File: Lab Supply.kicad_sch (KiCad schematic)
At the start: 56 parts, among them J1 V+, J2 V-, Q1 TIP121, Q2 2N3904, Q3 TIP121, Q5 2N3904, T1 115V to 24V, U1 LM324, U2 MCP4922, U3 LM7805, U4 LM4040DBZ-2.0, U6 MCP3202

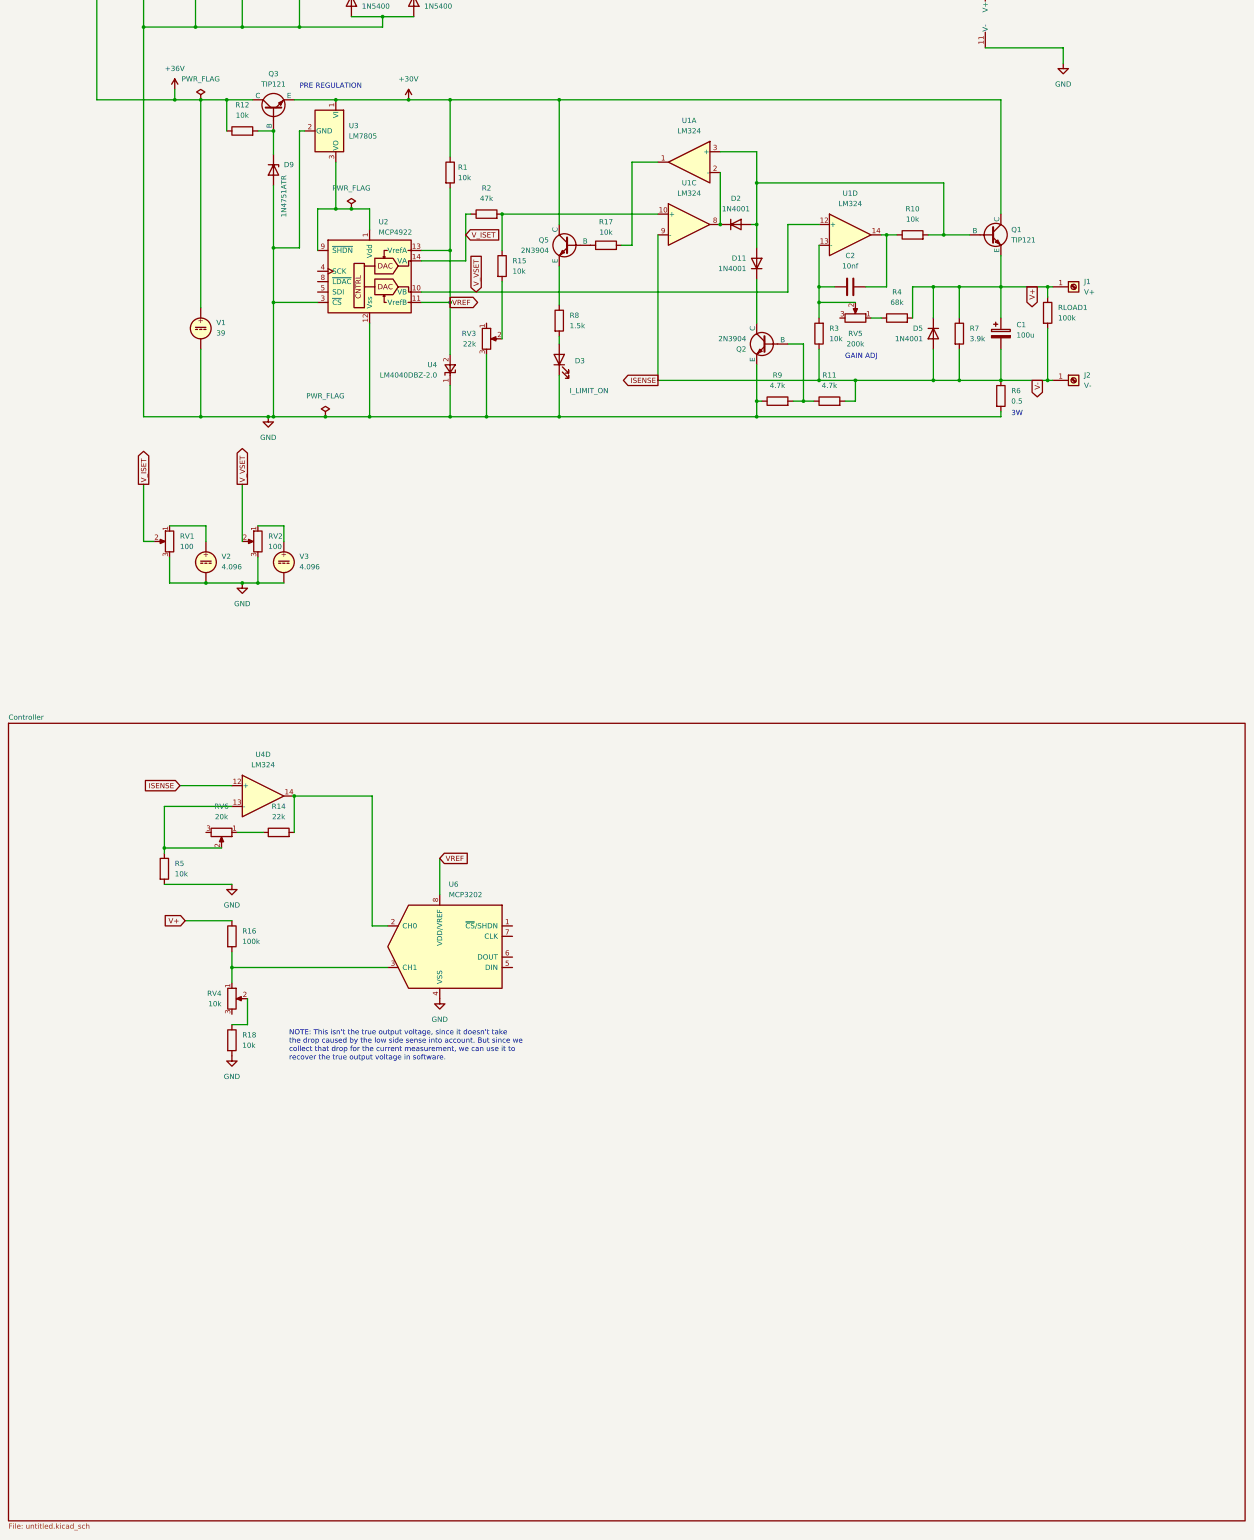
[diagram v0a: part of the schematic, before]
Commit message: Started working on firmware
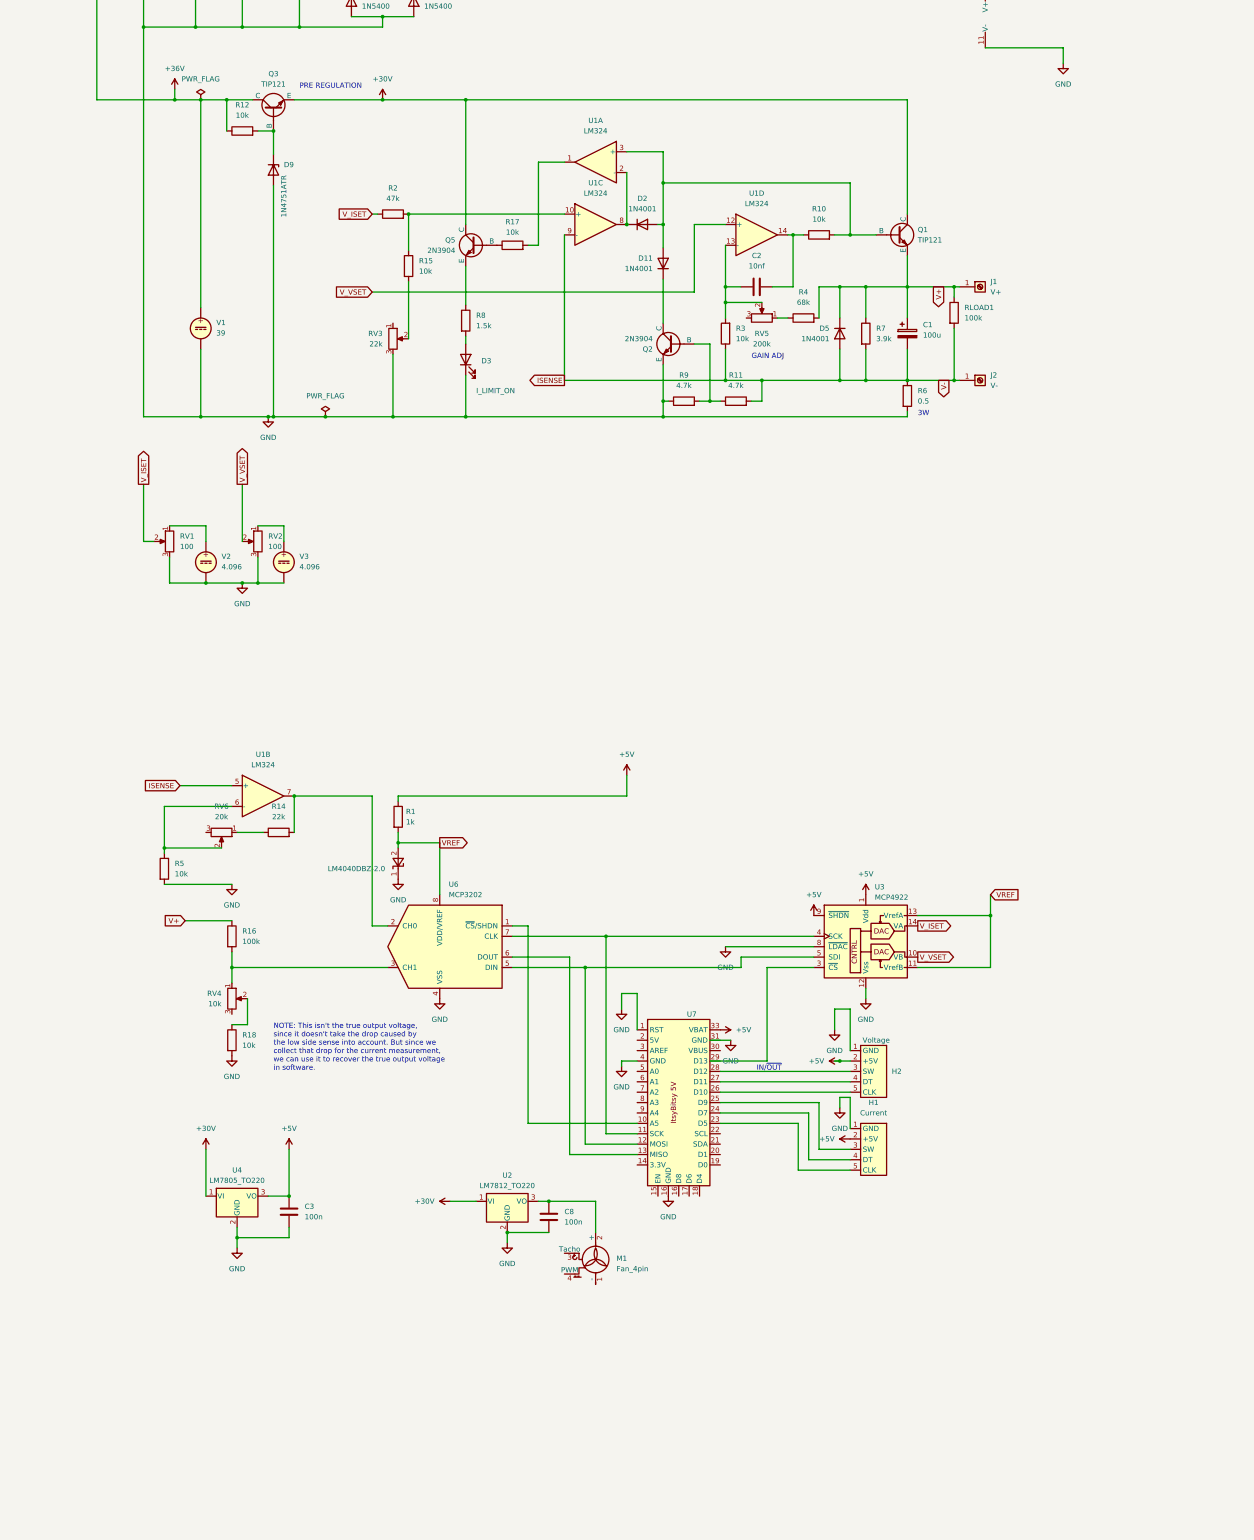
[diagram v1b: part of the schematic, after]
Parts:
- removed U2: MCP4922, Package_DIP:DIP-14_W7.62mm, symbol Analog_DAC:MCP4922
- removed U3: LM7805, Package_TO_SOT_THT:TO-220-3_Vertical, symbol Regulator_Linear:LM7805_TO220
- removed unit 1 of U4
- added C3: 100n, Capacitor_THT:C_Rect_L10.0mm_W2.5mm_P7.50mm_MKS4, symbol Device:C
- added C8: 100n, symbol Device:C
- added H1: Current, symbol Headers:Rotary_Header
- added H2: Voltage, symbol Headers:Rotary_Header
- added M1: Fan_4pin, symbol Motor:Fan_4pin
- added U2: LM7812_TO220, Package_TO_SOT_THT:TO-220-3_Vertical, symbol Regulator_Linear:LM7812_TO220
- added U3: MCP4922, Package_DIP:DIP-14_W7.62mm, symbol Analog_DAC:MCP4922
- added U4: LM7805_TO220, Package_TO_SOT_THT:TO-220-3_Vertical, symbol Regulator_Linear:LM7805_TO220
- added U5: LM4040DBZ-2.0, Package_TO_SOT_SMD:SOT-23, symbol Reference_Voltage:LM4040DBZ-2.0
- added U7: ~, Arduino:Itsy Bitsy 5V, symbol Arduino:ItsyBitsy_32u4-5V
- R1: value 10k -> 1k
- R14, R16, R18, R5: footprint (none) -> Resistor_THT:R_Axial_DIN0207_L6.3mm_D2.5mm_P2.54mm_Vertical
- RV3, RV4, RV6: footprint (none) -> Potentiometer_THT:Potentiometer_Bourns_3339H_Vertical
- RV5: footprint Resistor_THT:R_Axial_DIN0207_L6.3mm_D2.5mm_P2.54mm_Vertical -> Potentiometer_THT:Potentiometer_Bourns_3339H_Vertical
- U1: renamed from U4; footprint (none) -> Package_DIP:DIP-16_W7.62mm
- U6: footprint (none) -> Package_DIP:DIP-8_W7.62mm
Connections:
- net +28V: now also U2.1 (VI), U4.1 (VI); no longer R1.1
- net GND: now also C3.2, C8.2, H1.1 (GND), H2.1 (GND), U2.2 (GND), U3.12 (Vss), U3.8 (~{LDAC}), U4.2 (GND), U5.1 (K), U7.1 (RST), U7.16 (GND), U7.4 (GND)
- net ISENSE: now also U1.5 (+); no longer U1.12 (+)
- net VREF: now also U3.11 (VrefB), U3.13 (VrefA), U5.2 (A)
- net V_ISET: now also U3.14 (VA)
- net V_VSET: now also U3.10 (VB)
- net at R5.1, RV6.2: now also U1.6 (-); no longer U1.13 (-)
- net at R14.2, U6.2 (CH0): now also U1.7; no longer U1.14
- net at U6.1 (~{CS}/SHDN): now also U7.10 (A5)
- net at U6.5 (DIN): now also U3.5 (SDI), U7.12 (MOSI)
- net at U6.6 (DOUT): now also U7.13 (MISO)
- net at U6.7 (CLK): now also U3.4 (SCK), U7.11 (SCK)
- new net: C8.1, M1.2 (+), U2.3 (VO)
- new net: H1.3 (SW), U7.25 (D9)
- new net: H1.4 (DT), U7.24 (D7)
- new net: H1.5 (CLK), U7.23 (D5)
- new net: H2.5 (CLK), U7.26 (D10)
- new net: H2.4 (DT), U7.27 (D11)
- new net: H2.3 (SW), U7.28 (D12)
- new net +5V: C3.1, H1.2 (+5V), H2.2 (+5V), R1.1, U3.1 (Vdd), U3.9 (~{SHDN}), U4.3 (VO), U7.33 (VBAT)
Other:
- removed sheet Controller
- note added: "IN/~{OUT}"
- moved on the sheet: C1, C2, D11, D2, D3, D5, J1, J2, Q1, Q2, Q5, R10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

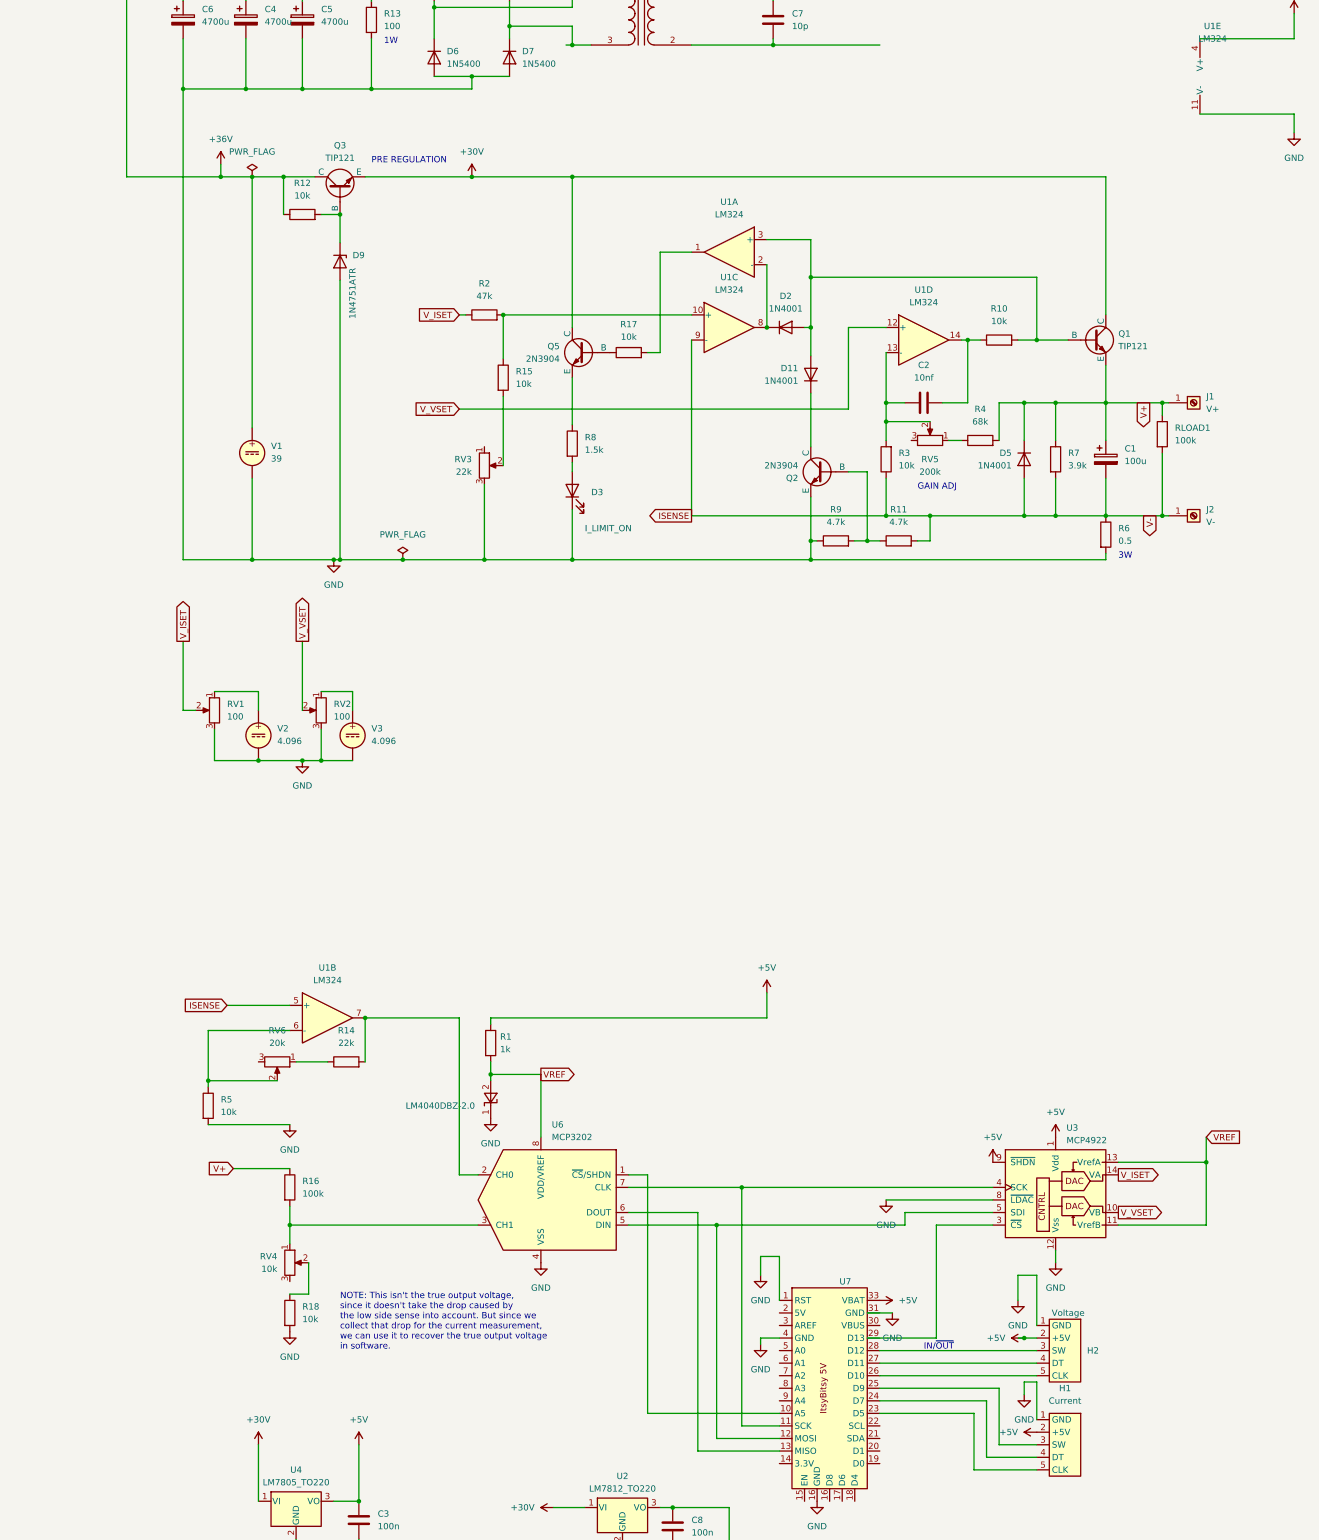
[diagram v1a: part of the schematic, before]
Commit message: WIP
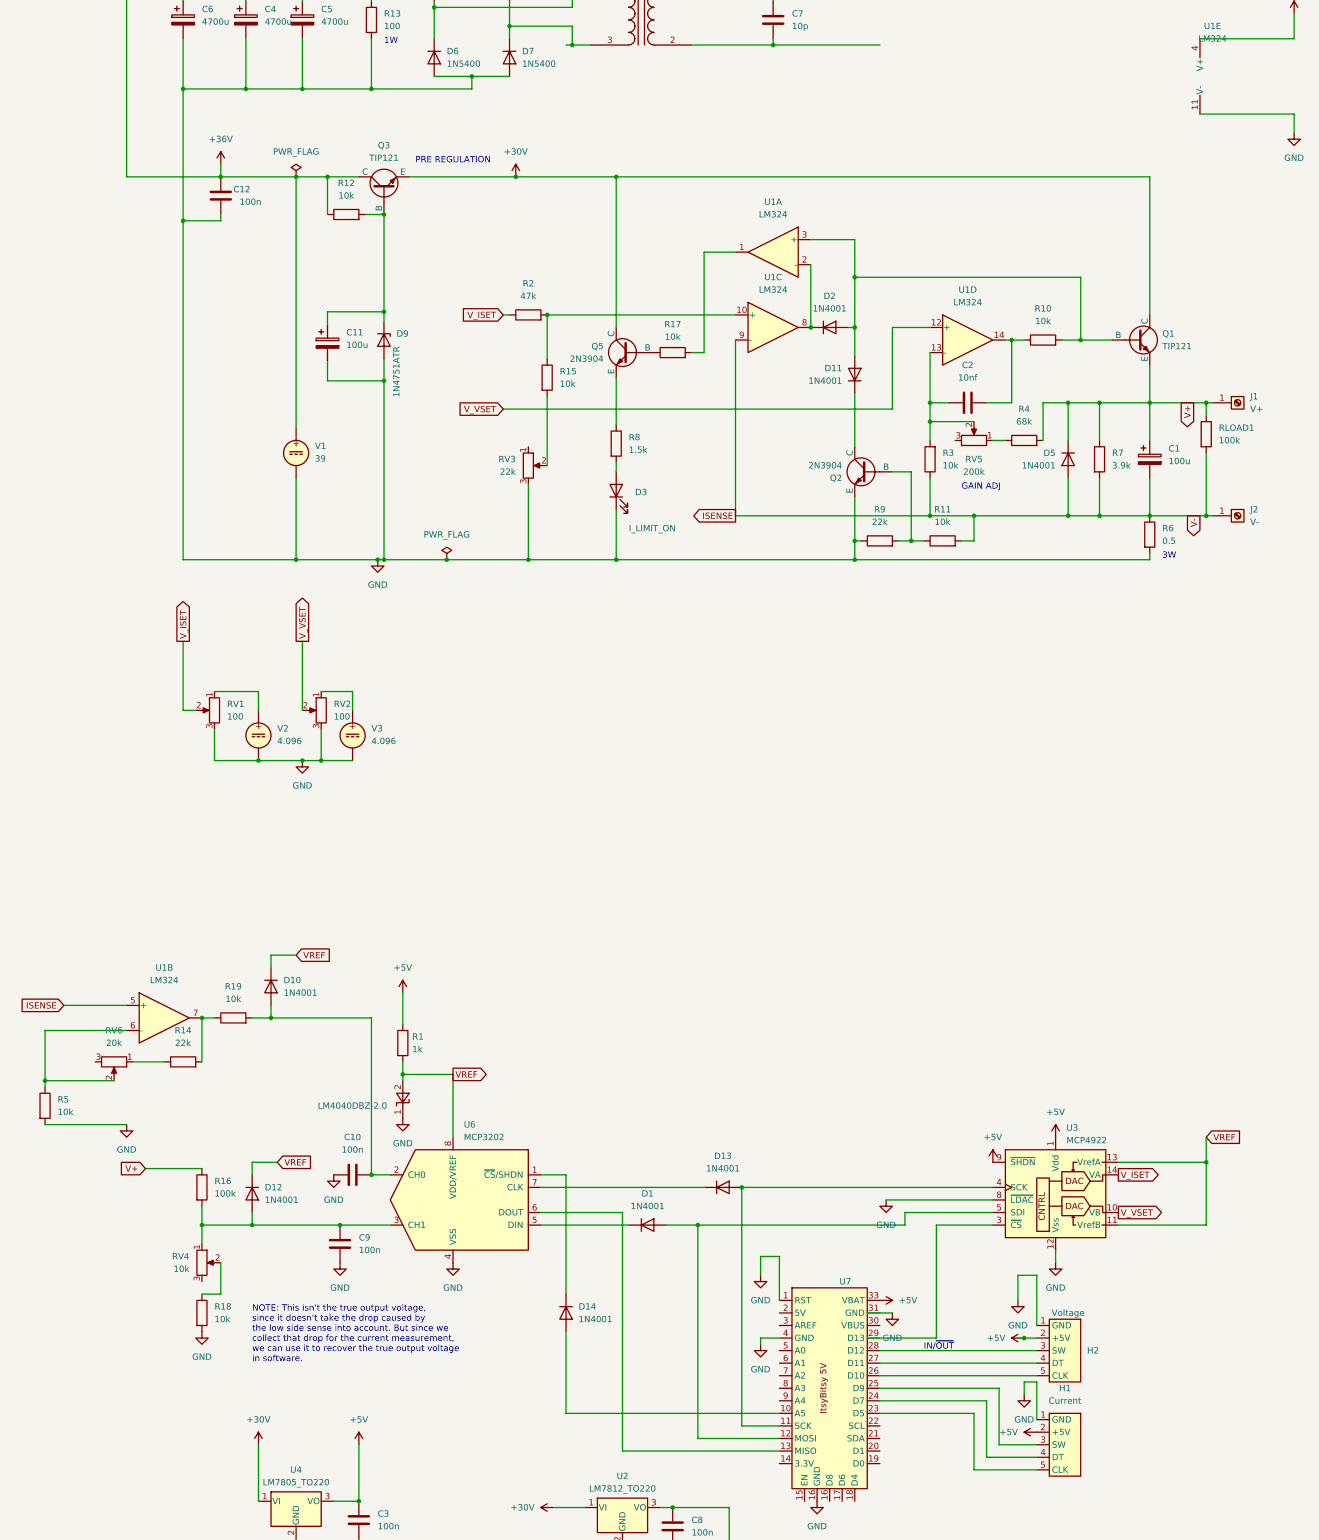
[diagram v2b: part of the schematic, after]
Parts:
- added C10, C12, C9: 100n, symbol Device:C
- added C11: 100u, symbol Device:C_Polarized
- added D1, D10, D12, D13, D14: 1N4001, symbol Device:D
- added R19: 10k, symbol Device:R
- R11: value 4.7k -> 10k
- R9: value 4.7k -> 22k
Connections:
- net +36V: now also C12.1
- net GND: now also C10.1, C11.2, C12.2, C9.2
- net VREF: now also D10.1 (K), D12.1 (K)
- net at U3.4 (SCK), U7.11 (SCK): now also D13.2 (A); no longer U6.7 (CLK)
- net at U3.5 (SDI), U7.12 (MOSI): now also D1.2 (A); no longer U6.5 (DIN)
- net at R14.2, U1.7: now also R19.1; no longer U6.2 (CH0)
- net at D9.1 (K), Q3.2 (B), R12.2: now also C11.1
- net at R16.2, RV4.1, U6.3 (CH1): now also C9.1, D12.2 (A)
- net at U6.1 (~{CS}/SHDN): now also D14.1 (K); no longer U7.10 (A5)
- new net: D14.2 (A), U7.10 (A5)
- new net: C10.2, D10.2 (A), R19.2, U6.2 (CH0)
- new net: D13.1 (K), U6.7 (CLK)
- new net: D1.1 (K), U6.5 (DIN)
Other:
- moved on the sheet: C1, C2, D11, D2, D3, D5, D9, J1, J2, Q1, Q2, Q3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
